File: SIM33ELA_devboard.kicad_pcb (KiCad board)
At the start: 4 copper layers, 40 x 24.9 mm, 13 parts, among them J2 Conn_01x13_Pin, U2 SIM33ELA

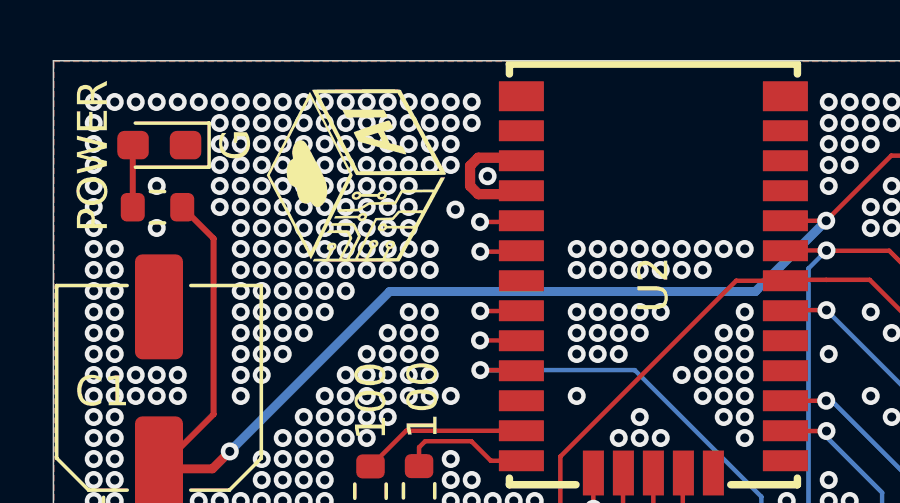
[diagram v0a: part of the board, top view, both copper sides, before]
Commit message: por si acaso
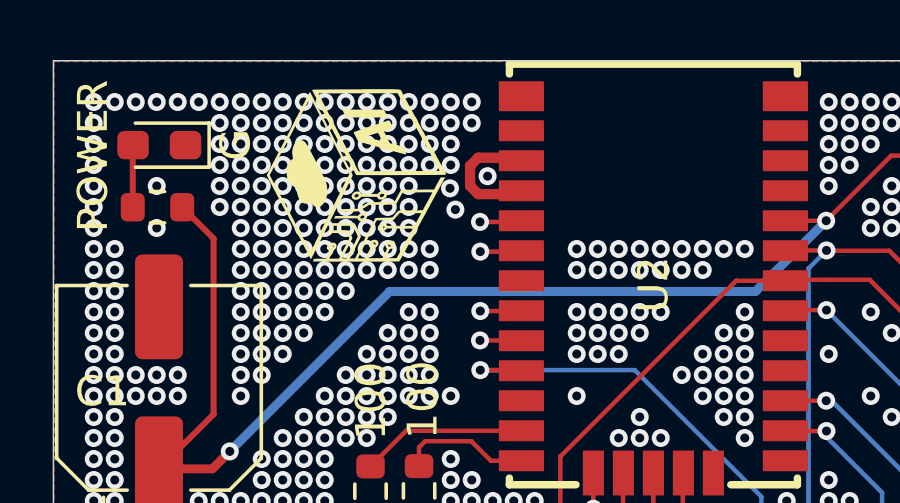
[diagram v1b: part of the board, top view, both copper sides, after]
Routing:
- net GND: vias 875 -> 876
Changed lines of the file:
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@@
+	)
+	(via
+		(at 137.99 85.11)
+		(size 0.6)
+		(drill 0.3)
+		(layers "F.Cu" "B.Cu")
+		(free yes)
+		(net 18)
 	)
 	(via
